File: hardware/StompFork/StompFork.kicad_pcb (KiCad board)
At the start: 2 copper layers, 100.3 x 58.4 mm, 32 parts, among them J1 Line-Level Input, J2 Direct Output, J3 Stompbox Output 1, J4 Stompbox Output 2, J5 Power, U1 TL074

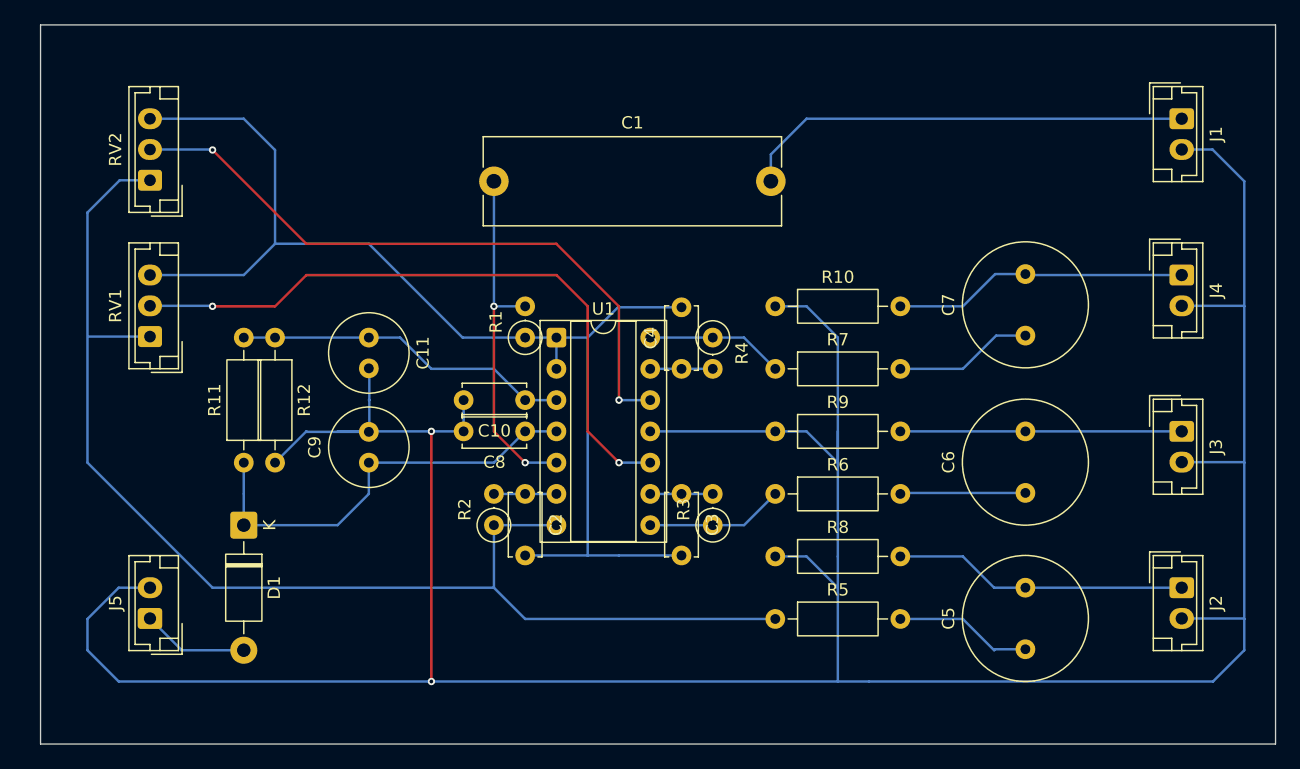
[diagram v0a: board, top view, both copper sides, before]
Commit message: Update PCB
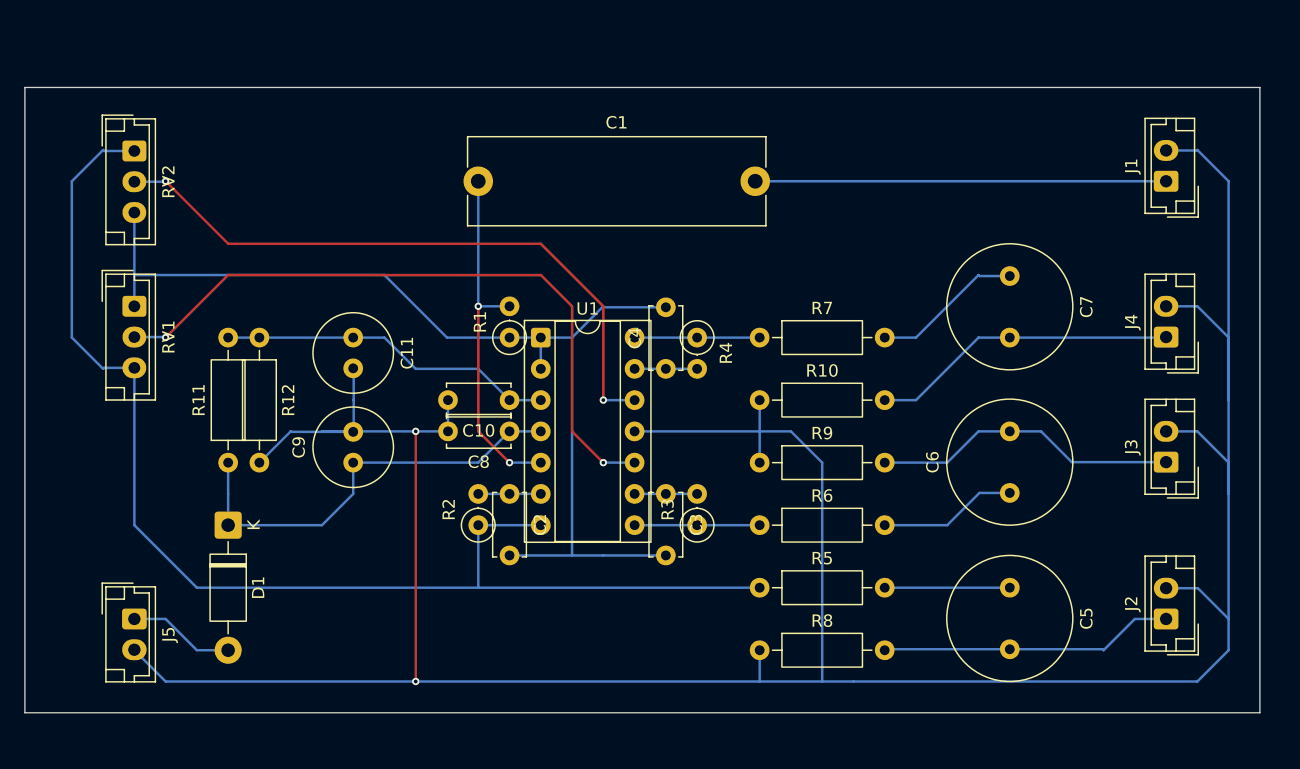
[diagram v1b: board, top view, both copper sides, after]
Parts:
- moved R8 7.73 mm to (160.0, 121.9)
- moved R10 7.73 mm to (160.0, 101.6)
- moved J1 5.24 mm to (193.0, 83.8), turned to 90 degrees
- moved J4 5.20 mm to (193.0, 96.5), turned to 90 degrees
- moved C5 5.16 mm to (180.3, 116.8), turned to -90 degrees
- moved C7 5.00 mm to (180.3, 91.5), turned to -90 degrees
- moved R6 2.84 mm to (160.0, 111.8)
- moved R7 2.84 mm to (160.0, 96.5)
- moved R9 2.84 mm to (160.0, 106.7)
- moved J2 2.84 mm to (193.0, 119.4), turned to 90 degrees
- moved R5 2.84 mm to (160.0, 116.8)
- moved J3 2.80 mm to (193.0, 106.6), turned to 90 degrees
- moved RV1 2.77 mm to (109.2, 94.0), turned to -90 degrees
- moved RV2 2.70 mm to (109.2, 81.4), turned to -90 degrees
- moved J5 1.27 mm to (109.2, 119.4), turned to -90 degrees
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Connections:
- RV1 pad 1: Net-(R2-Pad1) -> VREF
- RV1 pad 3: VREF -> Net-(R2-Pad1)
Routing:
- net GND: track 270.2 -> 249.9 mm
- net VREF: track 100.2 -> 86.9 mm
- net Net-(J1-T): track 36.8 -> 33.4 mm
- net Net-(J3-T): track 22.9 -> 24.9 mm
- net Net-(R2-Pad1): track 102.8 -> 100.9 mm
- net Net-(U1C-+): track 54.0 -> 55.1 mm
- net Net-(C5-Pad1): track 11.2 -> 10.2 mm
- net Net-(R4-Pad1): track 11.2 -> 10.2 mm
- net Net-(R3-Pad1): track 11.2 -> 10.2 mm
- net Net-(U1D-+): track 53.5 -> 52.5 mm
- net Net-(C6-Pad1): track 10.2 -> 11.2 mm
- net Net-(C7-Pad1): track 11.3 -> 12.3 mm
- net Net-(J4-T): track 24.0 -> 25.0 mm
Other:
- board size 100.3 x 58.4 mm -> 100.3 x 50.8 mm
